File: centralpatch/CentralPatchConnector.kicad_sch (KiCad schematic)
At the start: 1 part

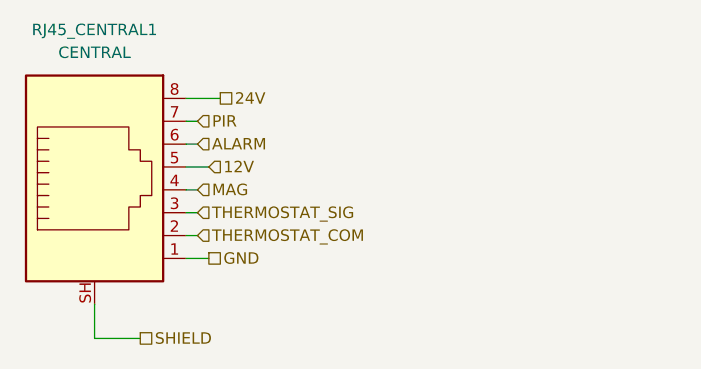
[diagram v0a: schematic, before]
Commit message: 20260607A
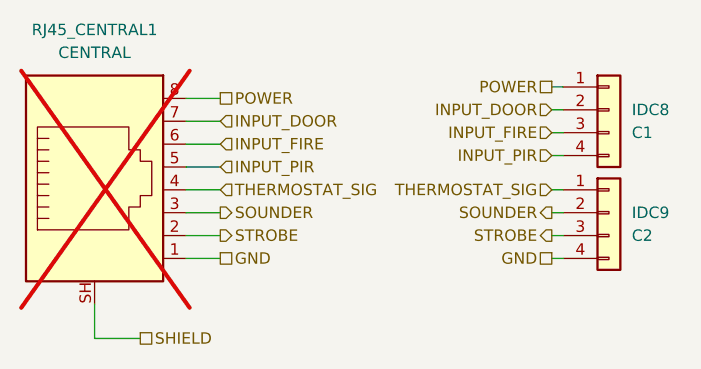
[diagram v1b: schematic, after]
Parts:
- added IDC8: C1, TerminalBlock_4Ucon:TerminalBlock_4Ucon_1x04_P3.50mm_Horizontal, symbol Connector_Generic:Conn_01x04
- added IDC9: C2, TerminalBlock_4Ucon:TerminalBlock_4Ucon_1x04_P3.50mm_Horizontal, symbol Connector_Generic:Conn_01x04
- RJ45_CENTRAL1: now not fitted; now left out of the parts list
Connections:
- net MAG is gone; now on net THERMOSTAT_SIG: RJ45_CENTRAL1.4
- net GND: now also IDC9.4 (Pin_4)
- net THERMOSTAT_SIG: now also IDC9.1 (Pin_1); no longer RJ45_CENTRAL1.3
- net 12V renamed INPUT_PIR
- net INPUT_PIR: now also IDC8.4 (Pin_4)
- net 24V renamed POWER
- net POWER: now also IDC8.1 (Pin_1)
- net ALARM renamed INPUT_FIRE
- net INPUT_FIRE: now also IDC8.3 (Pin_3)
- net PIR renamed INPUT_DOOR
- net INPUT_DOOR: now also IDC8.2 (Pin_2)
- net THERMOSTAT_COM renamed STROBE
- net STROBE: now also IDC9.3 (Pin_3)
- new net SOUNDER: IDC9.2 (Pin_2), RJ45_CENTRAL1.3
